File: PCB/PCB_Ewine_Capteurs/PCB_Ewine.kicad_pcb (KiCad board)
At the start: 2 copper layers, 25.9 x 22 mm, 17 parts, among them J2 Conn_2Rows-07Pins, M1 MLX90614ESF-AAA-000-TU, U1 VL53L3CXV0DH/1, U2 XC6206PxxxMR

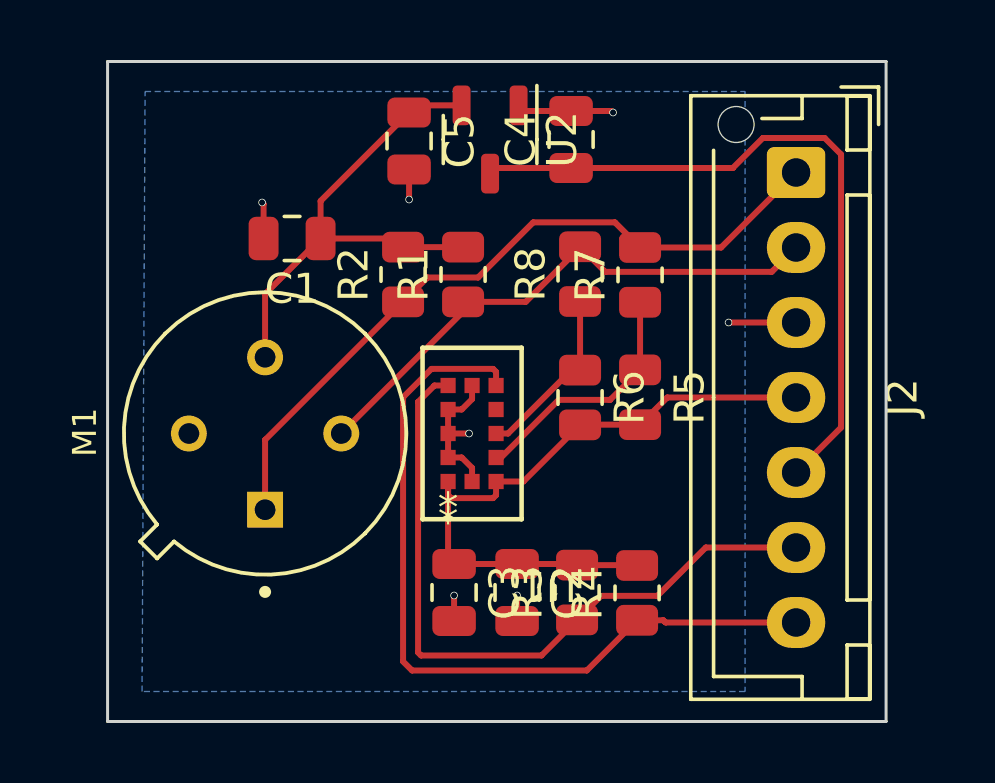
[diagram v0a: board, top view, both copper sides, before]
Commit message: wifi + pcb capteur fini + start pcb motherboard
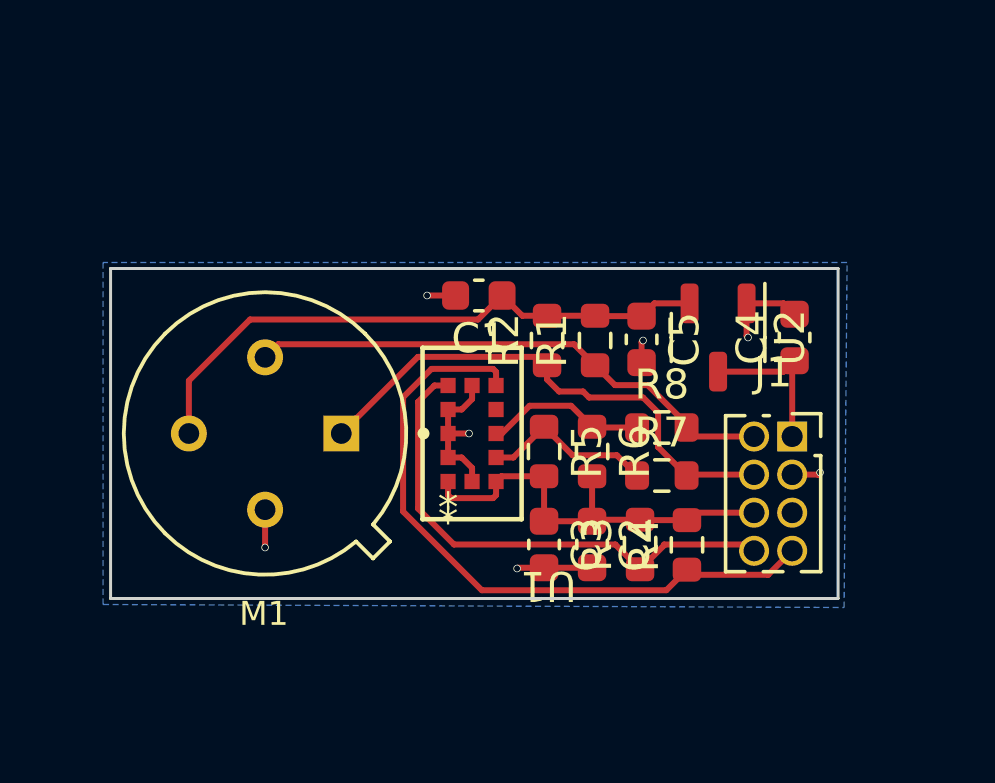
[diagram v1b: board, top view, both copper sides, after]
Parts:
- removed J2: Conn_2Rows-07Pins, Connector_JST:JST_XH_B7B-XH-AM_1x07_P2.50mm_Vertical
- added J1: Conn_01x08_Pin, Connector_PinSocket_1.27mm:PinSocket_2x04_P1.27mm_Vertical, F.Cu at (152.6, 46.5)
- C1, C2, C3, C4, C5: footprint Capacitor_SMD:C_0805_2012Metric -> Capacitor_SMD:C_0603_1608Metric
- R1, R2, R5, R6: footprint Resistor_SMD:R_0805_2012Metric -> Resistor_SMD:R_0603_1608Metric
- R3, R4: value 4.7K -> 10K; footprint Resistor_SMD:R_0805_2012Metric -> Resistor_SMD:R_0603_1608Metric
- R7, R8: value 4.7K -> 0; footprint Resistor_SMD:R_0805_2012Metric -> Resistor_SMD:R_0603_1608Metric
- moved C5 10.2 mm to (147.6, 43.3)
- moved U2 10.1 mm to (150.1, 43.2)
- moved C4 9.95 mm to (152.7, 43.2)
- moved R7 6.73 mm to (148.2, 47.8), turned to 0 degrees
- moved C1 6.51 mm to (142.1, 41.8)
- moved R8 5.79 mm to (148.2, 46.2), turned to 0 degrees
- moved R2 5.28 mm to (144.4, 43.3)
- moved R1 4.92 mm to (146.0, 43.3)
- moved R5 3.68 mm to (144.3, 47.0)
- moved C3 3.40 mm to (144.3, 50.1)
- moved C2 2.97 mm to (145.9, 50.1)
- moved R3 2.64 mm to (147.5, 50.1)
- moved R4 2.31 mm to (149.1, 50.1)
- moved R6 1.84 mm to (145.9, 47.0)
- turned M1 to 180 degrees
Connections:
- C2 pad 2: /GND_VL -> /GND
- C3 pad 2: /GND_VL -> /GND
- U1 pad 12: /GND_VL -> /GND
- U1 pad 2: /GND_VL -> /GND
- U1 pad 3: /GND_VL -> /GND
- U1 pad 4: /GND_VL -> /GND
- U1 pad 6: /GND_VL -> /GND
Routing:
- net /5V: track 23.6 -> 5.26 mm
- net /3.3V: track 23.1 -> 14.5 mm
- net /SCL: track 25.1 -> 17.7 mm
- net /GND_VL: track 6.79 -> 0.00 mm, vias 3 -> 0
- net /GND: track 7.72 -> 14.4 mm, vias 4 -> 7
- net /XSHUT: track 23.7 -> 17.3 mm
- net /GPIO_IRQ: track 26.7 -> 22.5 mm
- net /3.6V: track 16.9 -> 20.1 mm
- net /SCL_VL: track 8.48 -> 5.80 mm
- net /SDA: track 18.6 -> 17.8 mm
- net /SDA_VL: track 5.96 -> 5.38 mm
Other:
- board size 25.9 x 22 mm -> 24.2 x 11 mm
